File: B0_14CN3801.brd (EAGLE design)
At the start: 120 x 120 mm, 20 parts

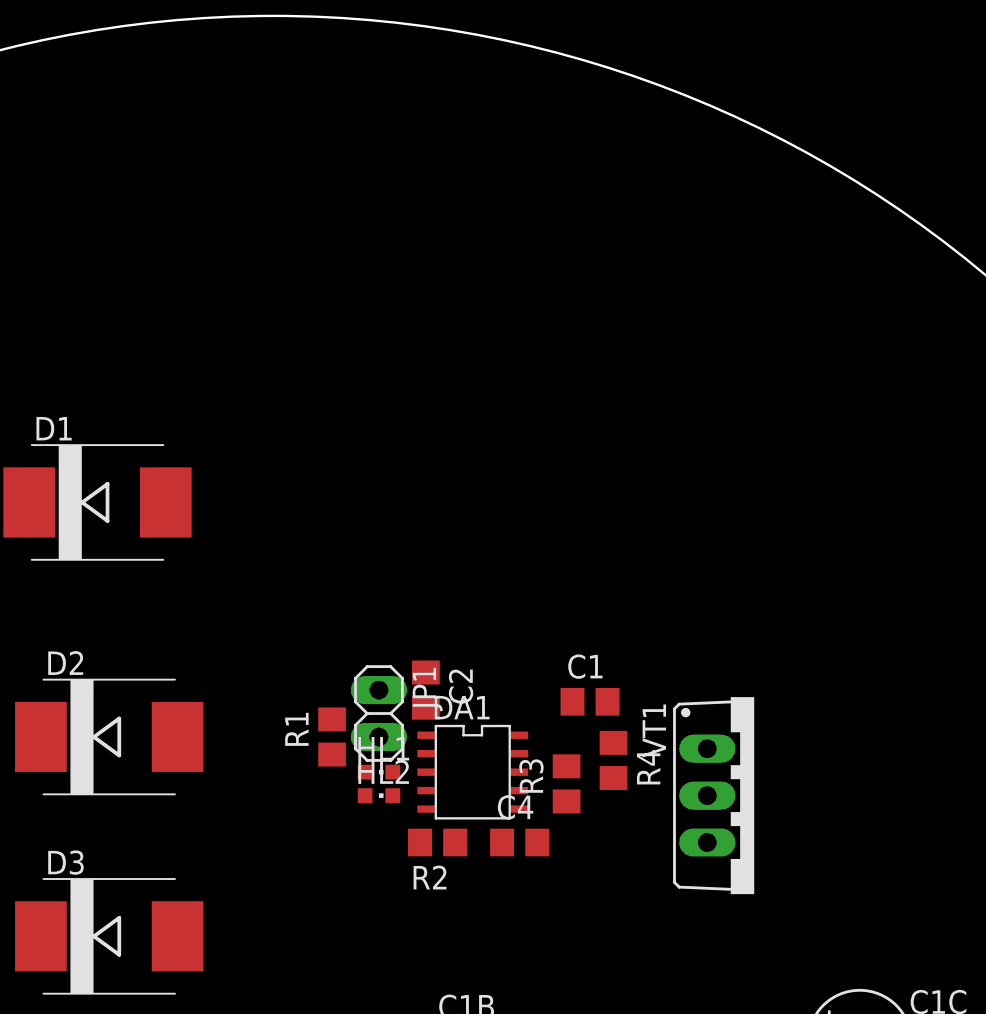
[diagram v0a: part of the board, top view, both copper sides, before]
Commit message: .
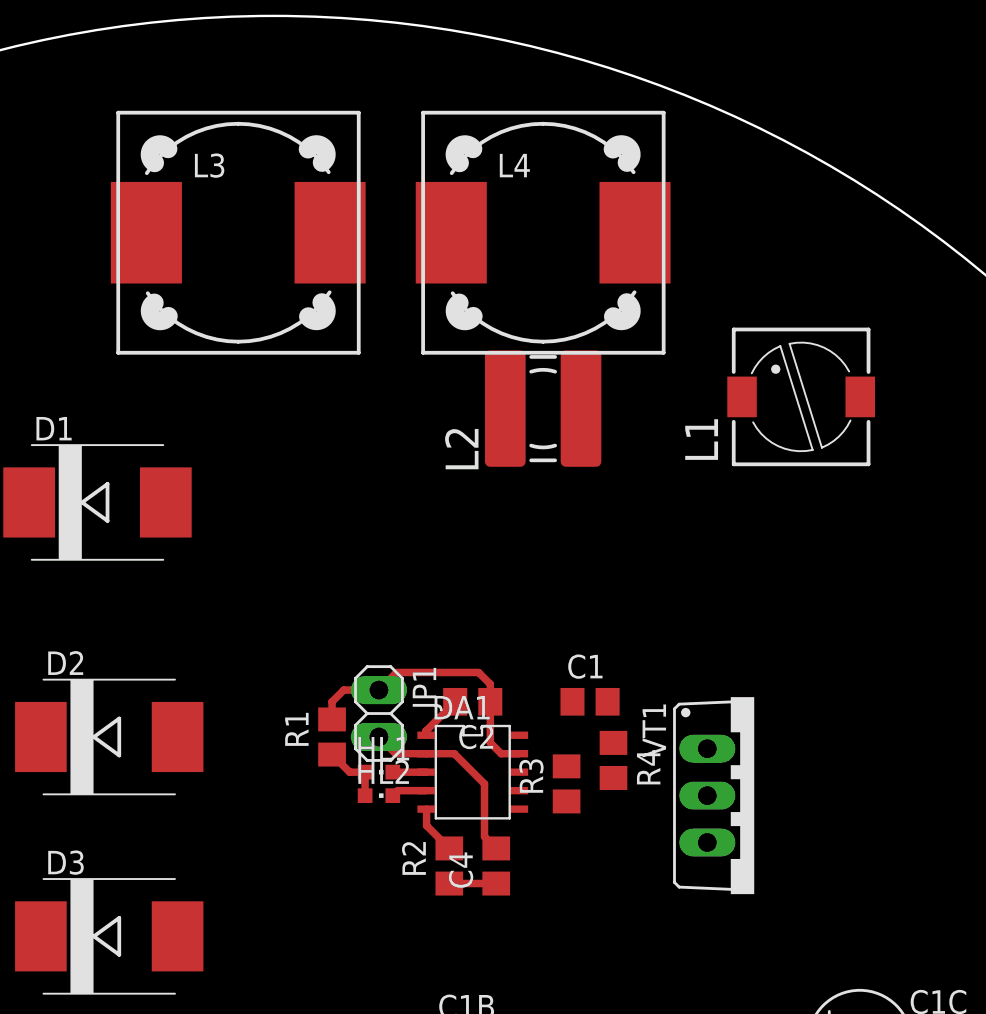
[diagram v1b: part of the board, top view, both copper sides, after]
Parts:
- added L1: (no value), rcl:PIS2816
- added L2: (no value), rcl:POWER-CHOKE_WE-TPC
- added L3: DR125, inductors:DR125
- added L4: DR127, inductors:DR127
- moved C2 2.62 mm to (62.2, 62.2), turned to 180 degrees
- moved C4 1.80 mm to (63.5, 53.3), turned to 90 degrees
- moved R2 1.42 mm to (61.0, 53.3), turned to 90 degrees
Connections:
- net N$4 renamed COM
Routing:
- net N$1: track 0.00 -> 15.4 mm
- net GND: track 0.00 -> 10.5 mm
- net N$5: track 0.00 -> 3.46 mm
- net COM: track 0.00 -> 2.64 mm
- net N$8: track 0.00 -> 2.54 mm
- net N$2: track 0.00 -> 2.49 mm
- net N$7: track 0.00 -> 1.94 mm
- net N$6: track 0.00 -> 1.83 mm
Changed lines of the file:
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@@
 <dimension x1="53.34" y1="44.45" x2="77.47" y2="41.275" x3="65.405" y3="76.835" textsize="1.778" layer="47" dtype="horizontal"/>
 <dimension x1="42.545" y1="65.405" x2="45.72" y2="51.435" x3="90.805" y3="58.42" textsize="1.778" layer="47" dtype="vertical"/>
+<dimension x1="43.18" y1="94.615" x2="55.88" y2="94.615" x3="49.53" y3="101.6" textsize="1.778" layer="1" dtype="horizontal"/>
+<dimension x1="76.2" y1="81.915" x2="83.82" y2="81.915" x3="80.01" y3="87.63" textsize="1.778" layer="1" dtype="horizontal"/>
 </plain>
 <attributes>
@@
 <elements>
 <element name="DA1" library="Consonance" package="SSOP10" value="CN3801" x="62.23" y="58.42"/>
-<element name="C2" library="rcl" package="C0805" value="100n" x="59.69" y="62.865" rot="R270"/>
+<element name="C2" library="rcl" package="C0805" value="100n" x="62.23" y="62.23" rot="R180"/>
 <element name="C1" library="rcl" package="C0805" value="100n" x="68.58" y="62.23"/>
 <element name="HL1" library="led" package="CHIPLED_0603" value="" x="57.15" y="58.42" rot="R270"/>
 <element name="HL2" library="led" package="CHIPLED_0603" value="" x="57.15" y="57.15" rot="R270"/>
 <element name="R1" library="rcl" package="R0805" value="" x="54.61" y="60.325" rot="R90"/>
-<element name="R2" library="rcl" package="R0805" value="120" x="60.325" y="54.61" rot="R180"/>
+<element name="R2" library="rcl" package="R0805" value="120" x="60.96" y="53.34" rot="R90"/>
 <element name="R3" library="rcl" package="R0805" value="" x="67.31" y="57.785" rot="R90"/>
 <element name="R4" library="rcl" package="R0805" value="" x="69.85" y="59.055" rot="R270"/>
-<element name="C4" library="rcl" package="C0805" value="220n" x="64.77" y="54.61"/>
+<element name="C4" library="rcl" package="C0805" value="220n" x="63.5" y="53.34" rot="R90"/>
 <element name="VT1" library="m_transistor" package="TO220FV" value="" x="77.47" y="57.15" rot="R270"/>
 <element name="JP1" library="Разъёмы штырьковые 2.54мм" package="1X02" value="" x="57.15" y="61.595" rot="R270"/>
@@
 <element name="D3" library="diode" package="SMC" value="" x="42.545" y="49.53"/>
 <element name="U$1" library="B0_14CN3801" package="PCB1" value="" x="51.435" y="39.37"/>
+<element name="L1" library="rcl" package="PIS2816" value="" x="80.01" y="78.74" rot="R90"/>
+<element name="L2" library="rcl" package="POWER-CHOKE_WE-TPC" value="" x="66.04" y="78.105" rot="R90"/>
+<element name="L3" library="inductors" package="DR125" value="DR125" x="49.53" y="87.63"/>
+<element name="L4" library="inductors" package="DR127" value="DR127" x="66.04" y="87.63"/>
 </elements>
 <signals>
@@
 <contactref element="DA1" pad="1"/>
 <contactref element="C2" pad="2"/>
-<wire x1="59.73" y1="60.42" x2="59.69" y2="61.915" width="0" layer="19" extent="1-1"/>
+<wire x1="59.69" y1="60.46" x2="59.73" y2="60.42" width="0.4064" layer="1"/>
+<wire x1="59.69" y1="60.46" x2="59.69" y2="60.64" width="0.4064" layer="1"/>
+<wire x1="59.69" y1="60.64" x2="61.28" y2="62.23" width="0.4064" layer="1"/>
 </signal>
 <signal name="GND">
@@
 <contactref element="C3" pad="-"/>
 <wire x1="69.85" y1="60.005" x2="69.53" y2="62.23" width="0" layer="19" extent="1-1"/>
-<wire x1="65.72" y1="54.61" x2="69.85" y2="60.005" width="0" layer="19" extent="1-1"/>
-<wire x1="59.73" y1="59.42" x2="65.72" y2="54.61" width="0" layer="19" extent="1-1"/>
-<wire x1="57.15" y1="60.325" x2="59.73" y2="59.42" width="0" layer="19" extent="1-1"/>
-<wire x1="72.39" y1="41.91" x2="65.72" y2="54.61" width="0" layer="19" extent="1-1"/>
+<wire x1="63.5" y1="54.29" x2="69.85" y2="60.005" width="0" layer="19" extent="1-1"/>
+<wire x1="72.39" y1="41.91" x2="63.5" y2="54.29" width="0" layer="19" extent="1-1"/>
 <wire x1="74.61" y1="36.195" x2="72.39" y2="41.91" width="0" layer="19" extent="1-1"/>
+<wire x1="59.73" y1="59.42" x2="61.23" y2="59.42" width="0.4064" layer="1"/>
+<wire x1="61.23" y1="59.42" x2="62.865" y2="57.785" width="0.4064" layer="1"/>
+<wire x1="62.865" y1="57.785" x2="62.865" y2="54.925" width="0.4064" layer="1"/>
+<wire x1="62.865" y1="54.925" x2="63.5" y2="54.29" width="0.4064" layer="1"/>
+<wire x1="59.73" y1="59.42" x2="58.055" y2="59.42" width="0.4064" layer="1"/>
+<wire x1="58.055" y1="59.42" x2="57.15" y2="60.325" width="0.4064" layer="1"/>
 </signal>
 <signal name="N$5">
@@
 <contactref element="HL2" pad="A"/>
 <contactref element="HL1" pad="A"/>
-<wire x1="56.4" y1="57.15" x2="56.4" y2="58.42" width="0" layer="19" extent="1-1"/>
-<wire x1="54.61" y1="59.375" x2="56.4" y2="58.42" width="0" layer="19" extent="1-1"/>
+<wire x1="56.4" y1="57.15" x2="56.4" y2="58.42" width="0.4064" layer="1"/>
+<wire x1="56.4" y1="58.42" x2="55.565" y2="58.42" width="0.4064" layer="1"/>
+<wire x1="55.565" y1="58.42" x2="54.61" y2="59.375" width="0.4064" layer="1"/>
 </signal>
 <signal name="N$6">
 <contactref element="HL1" pad="C"/>
 <contactref element="DA1" pad="3"/>
-<wire x1="57.9" y1="58.42" x2="59.73" y2="58.42" width="0" layer="19" extent="1-1"/>
+<wire x1="57.9" y1="58.42" x2="59.73" y2="58.42" width="0.4064" layer="1"/>
 </signal>
 <signal name="N$7">
 <contactref element="HL2" pad="C"/>
 <contactref element="DA1" pad="4"/>
-<wire x1="57.9" y1="57.15" x2="59.73" y2="57.42" width="0" layer="19" extent="1-1"/>
+<wire x1="59.73" y1="57.42" x2="58.17" y2="57.42" width="0.4064" layer="1"/>
+<wire x1="58.17" y1="57.42" x2="57.9" y2="57.15" width="0.4064" layer="1"/>
 </signal>
 <signal name="N$3">
@@
 <wire x1="64.73" y1="56.42" x2="67.31" y2="56.835" width="0" layer="19" extent="1-1"/>
 </signal>
-<signal name="N$4">
+<signal name="COM">
 <contactref element="DA1" pad="5"/>
 <contactref element="R2" pad="2"/>
-<wire x1="59.375" y1="54.61" x2="59.73" y2="56.42" width="0" layer="19" extent="1-1"/>
+<wire x1="59.73" y1="56.42" x2="59.73" y2="55.52" width="0.4064" layer="1"/>
+<wire x1="59.73" y1="55.52" x2="60.96" y2="54.29" width="0.4064" layer="1"/>
 </signal>
 <signal name="N$8">
 <contactref element="R2" pad="1"/>
 <contactref element="C4" pad="1"/>
-<wire x1="61.275" y1="54.61" x2="63.82" y2="54.61" width="0" layer="19" extent="1-1"/>
+<wire x1="60.96" y1="52.39" x2="63.5" y2="52.39" width="0.4064" layer="1"/>
 </signal>
 <signal name="N$9">
@@
 <wire x1="67.31" y1="58.735" x2="67.63" y2="62.23" width="0" layer="19" extent="1-1"/>
 <wire x1="64.73" y1="59.42" x2="67.31" y2="58.735" width="0" layer="19" extent="1-1"/>
-<wire x1="59.69" y1="63.815" x2="64.73" y2="59.42" width="0" layer="19" extent="1-1"/>
-<wire x1="57.15" y1="62.865" x2="59.69" y2="63.815" width="0" layer="19" extent="1-1"/>
-<wire x1="54.61" y1="61.275" x2="57.15" y2="62.865" width="0" layer="19" extent="1-1"/>
 <wire x1="74.93" y1="54.61" x2="67.31" y2="58.735" width="0" layer="19" extent="1-1"/>
+<wire x1="58.1" y1="63.815" x2="57.15" y2="62.865" width="0.4064" layer="1"/>
+<wire x1="57.15" y1="62.865" x2="55.245" y2="62.865" width="0.4064" layer="1"/>
+<wire x1="55.245" y1="62.865" x2="54.61" y2="62.23" width="0.4064" layer="1"/>
+<wire x1="54.61" y1="62.23" x2="54.61" y2="61.275" width="0.4064" layer="1"/>
+<wire x1="64.73" y1="59.42" x2="63.77" y2="59.42" width="0.4064" layer="1"/>
+<wire x1="63.18" y1="62.23" x2="63.18" y2="60.01" width="0.4064" layer="1"/>
+<wire x1="63.18" y1="60.01" x2="63.77" y2="59.42" width="0.4064" layer="1"/>
+<wire x1="58.1" y1="63.815" x2="62.55" y2="63.815" width="0.4064" layer="1"/>
+<wire x1="63.18" y1="62.23" x2="63.18" y2="63.185" width="0.4064" layer="1"/>
+<wire x1="63.18" y1="63.185" x2="62.55" y2="63.815" width="0.4064" layer="1"/>
 </signal>
 <signal name="N$10">
